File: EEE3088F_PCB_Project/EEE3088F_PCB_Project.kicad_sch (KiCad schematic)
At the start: 69 parts, among them IC1 DRV8833PWPR, IC2 DRV8833PWPR, IC3 TPS62067DSGR, IC5 INA219AIDCNR, IC7 TPS61088RHLR, J1 Conn_02x16_Odd_Even, J2 TYPE-C16PIN, J3 Conn_01x02, Q1 AO3400A, Q2 AO3400A, Q5 AO3401A, Q6 AO3401A, SW1 1MS1T1B1M2QES, U1 HUSB237-AA001-DN06R, U2 SLM6600, U3 IRLML6344TRPBF

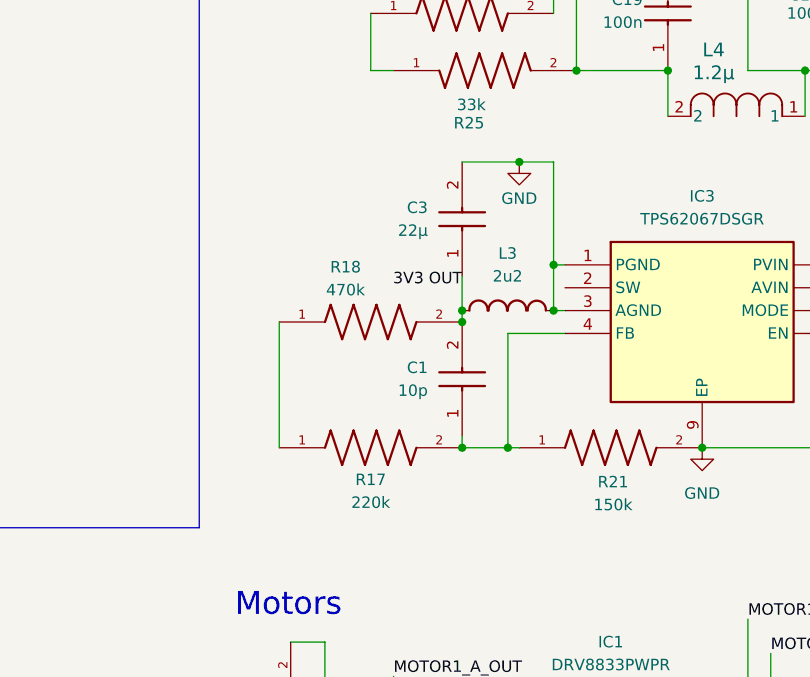
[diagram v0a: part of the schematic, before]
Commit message: v1.2
Starting with PCB design
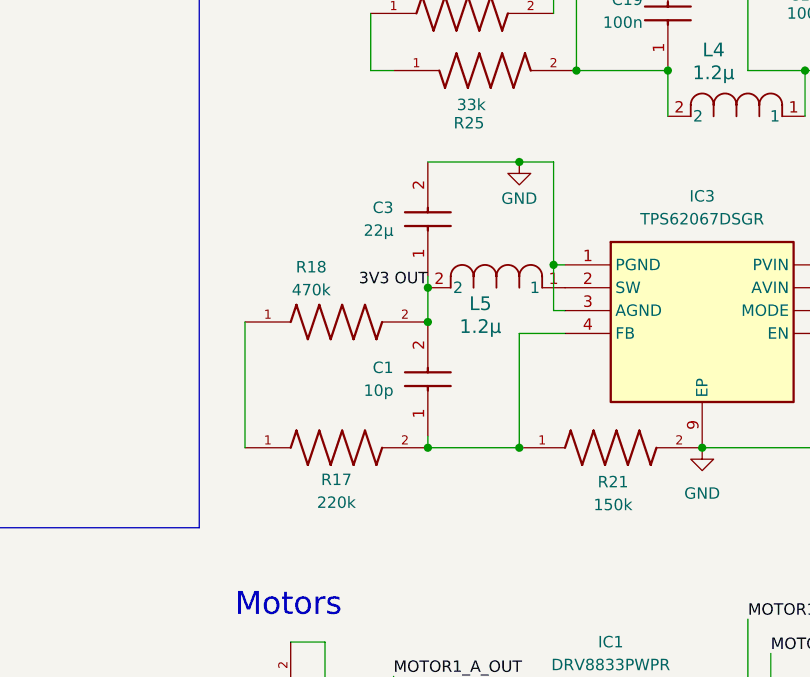
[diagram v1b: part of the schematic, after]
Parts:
- removed L3: 2u2, symbol FHW0805UF2R2JST:FHW0805UF2R2JST
- added L5: 1.2µ, IND_FXL0420_CMT, symbol 2025-03-28_01-51-26:FXL0420-6R8-M
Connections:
- net 3V3 OUT: now also L5.2
- net at IC3.2 (SW): now also L5.1
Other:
- moved on the sheet: C1, C3, R17, R18
